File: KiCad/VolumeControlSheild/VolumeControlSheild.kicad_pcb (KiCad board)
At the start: 2 copper layers, 68.6 x 53.3 mm, 30 parts, among them J1 Power, J2 Digital/PWM, J3 Analog, J4 Digital/PWM, J5 Conn_01x08, SW1 EC11E15204A3, U1 TSOP4838(?), U2 TSOP7000, U3 OLED SSH1106, U4 LM317_TO-252

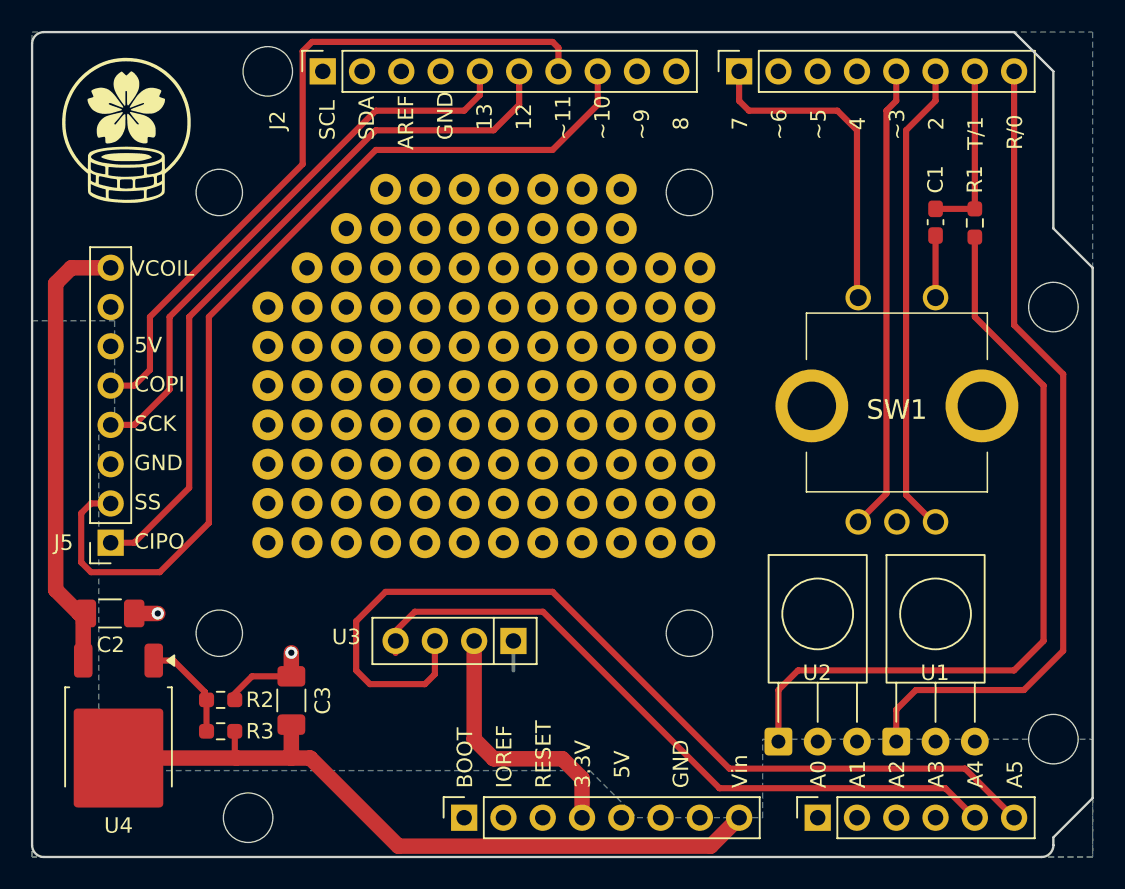
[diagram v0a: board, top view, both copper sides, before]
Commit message: Gerber generated.
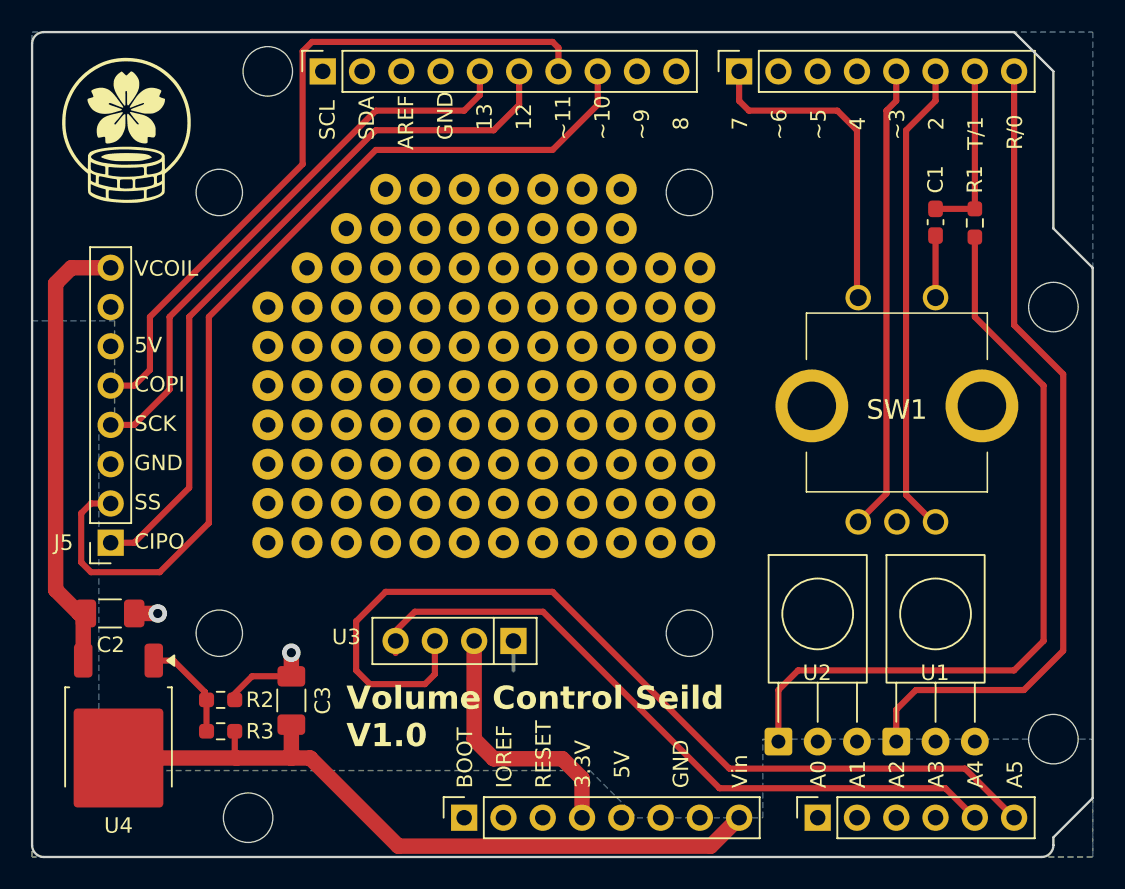
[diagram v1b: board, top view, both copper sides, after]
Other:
- board text added: "Volume Control Seild V1.0"
